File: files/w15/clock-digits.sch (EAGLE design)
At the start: 6 parts, among them IC1 ATTINY44-SSU, IC2 5V

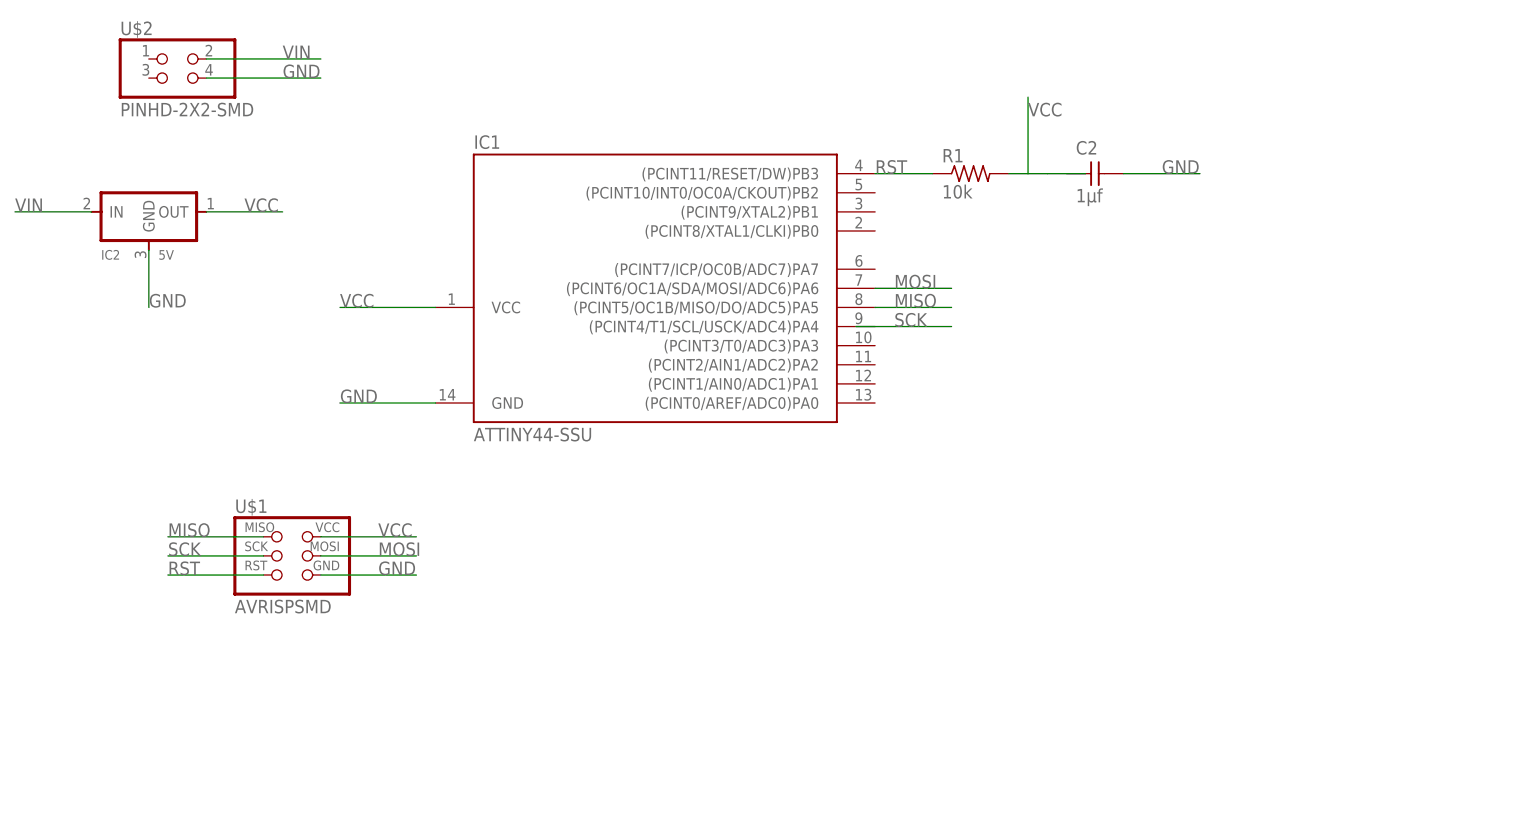
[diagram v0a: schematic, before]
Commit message: board routing
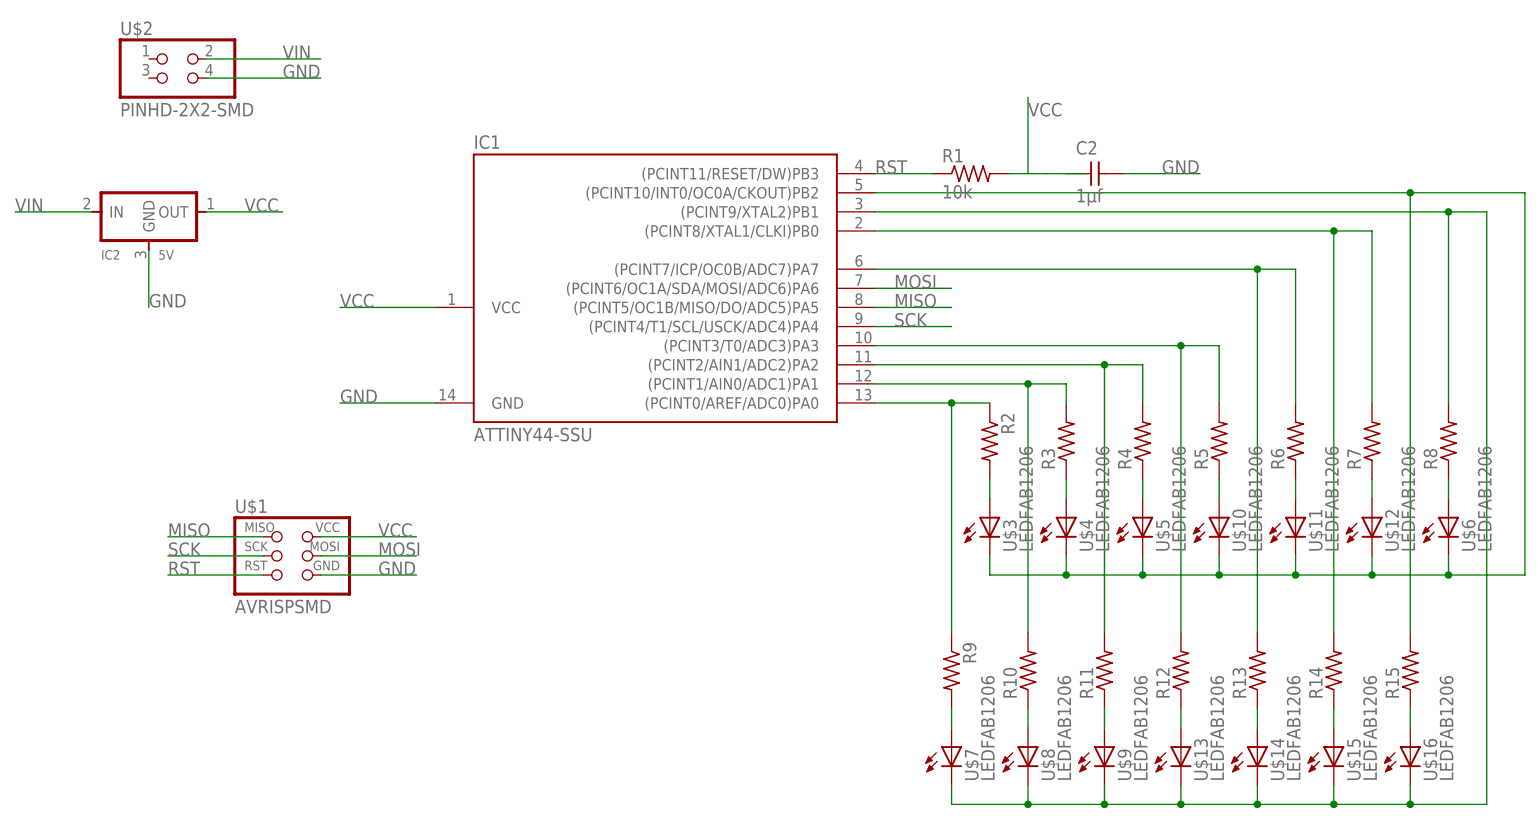
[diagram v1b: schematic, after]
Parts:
- added R10, R11, R12, R13, R14, R15, R2, R3, R4, R5, R6, R7, R8, R9: (no value), fab:RES-US1206FAB
- added U$10, U$11, U$12, U$13, U$14, U$15, U$16, U$3, U$4, U$5, U$6, U$7, U$8, U$9: LEDFAB1206, fab:LEDFAB1206
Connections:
- new net N$1: IC1.(PCINT0/AREF/ADC0)PA0, R2.1, R9.1
- new net N$10: R6.1, U$11.A
- new net N$11: IC1.(PCINT8/XTAL1/CLKI)PB0, R14.2, R7.2
- new net N$12: R7.1, U$12.A
- new net N$14: R8.1, U$6.A
- new net N$15: IC1.(PCINT10/INT0/OC0A/CKOUT)PB2, R15.2, U$10.C, U$11.C, U$12.C, U$3.C, U$4.C, U$5.C, U$6.C
- new net N$16: R9.2, U$7.A
- new net N$17: R15.1, U$16.A
- new net N$18: R10.1, U$8.A
- new net N$2: R2.2, U$3.A
- new net N$20: R11.1, U$9.A
- new net N$21: R12.1, U$13.A
- new net N$23: R13.1, U$14.A
- new net N$24: R14.1, U$15.A
- new net N$28: IC1.(PCINT9/XTAL2)PB1, R8.2, U$13.C, U$14.C, U$15.C, U$16.C, U$7.C, U$8.C, U$9.C
- new net N$3: IC1.(PCINT1/AIN0/ADC1)PA1, R10.2, R3.2
- new net N$4: R3.1, U$4.A
- new net N$5: IC1.(PCINT2/AIN1/ADC2)PA2, R11.2, R4.2
- new net N$6: R4.1, U$5.A
- new net N$7: IC1.(PCINT3/T0/ADC3)PA3, R12.2, R5.2
- new net N$8: R5.1, U$10.A
- new net N$9: IC1.(PCINT7/ICP/OC0B/ADC7)PA7, R13.2, R6.2
- net SCK: now also IC1.(PCINT4/T1/SCL/USCK/ADC4)PA4
